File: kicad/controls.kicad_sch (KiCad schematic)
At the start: 5 parts, among them P1 Potentiometer_9mm_Vertical_Li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, P2 Potentiometer_9mm_Vertical_Li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, SW1 SW_Push_LED, SW2 SW_Push_LED, U7 ADC121C027CIMK

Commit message: reroute pcb
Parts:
- P1, P2: footprint Eurorack:Potentiometer 9mm Vertical Linear Centred -> allen-synthesis:potentiometer-9mm
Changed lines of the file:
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@@
       (effects (font (size 1.27 1.27)) (justify right) hide)
     )
-    (property "Footprint" "Eurorack:Potentiometer 9mm Vertical Linear Centred" (at 27.94 34.29 0)
+    (property "Footprint" "allen-synthesis:potentiometer-9mm" (at 27.94 34.29 0)
       (effects (font (size 1.27 1.27)) hide)
     )
@@
       (effects (font (size 1.27 1.27)) (justify right) hide)
     )
-    (property "Footprint" "Eurorack:Potentiometer 9mm Vertical Linear Centred" (at 59.69 34.29 0)
+    (property "Footprint" "allen-synthesis:potentiometer-9mm" (at 59.69 34.29 0)
       (effects (font (size 1.27 1.27)) hide)
     )

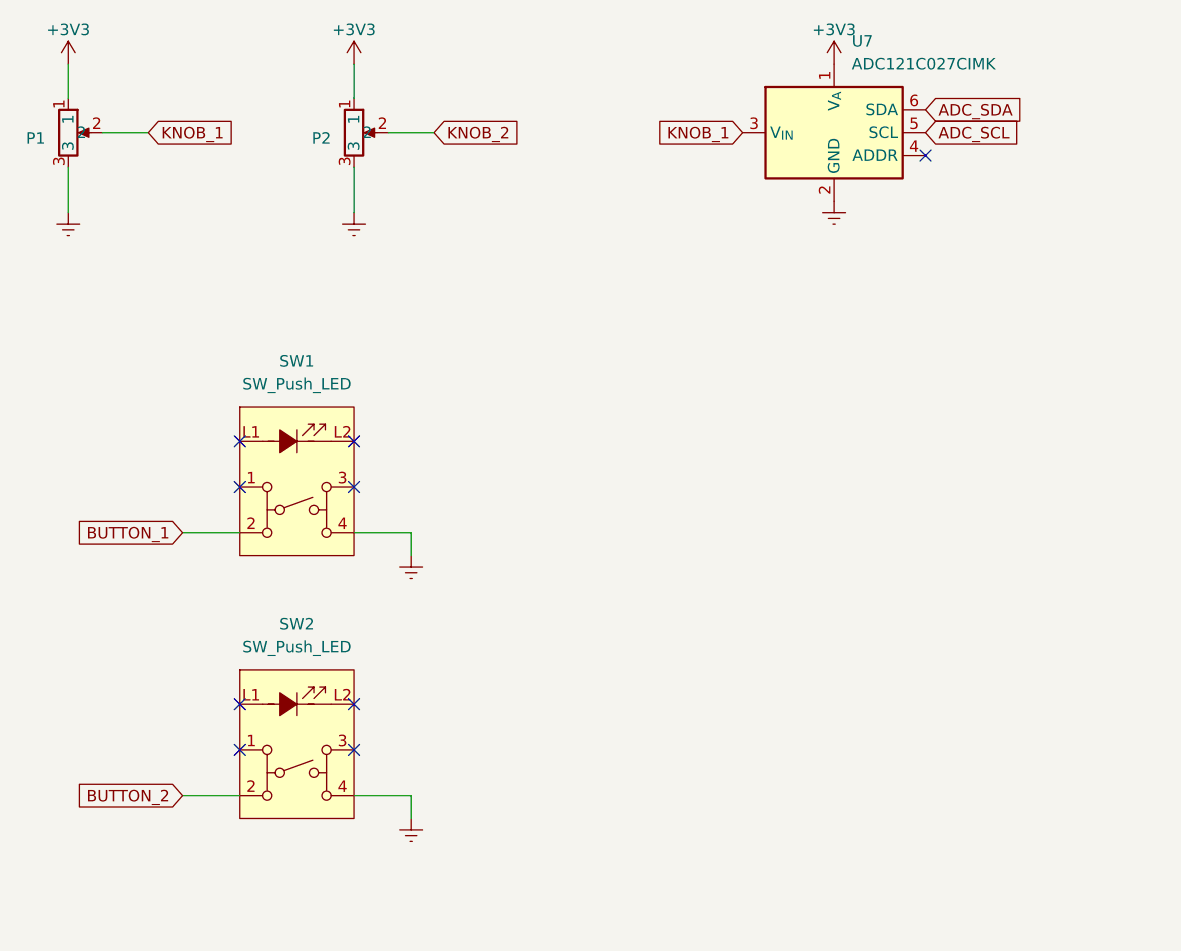
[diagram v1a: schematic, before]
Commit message: add schematic notes
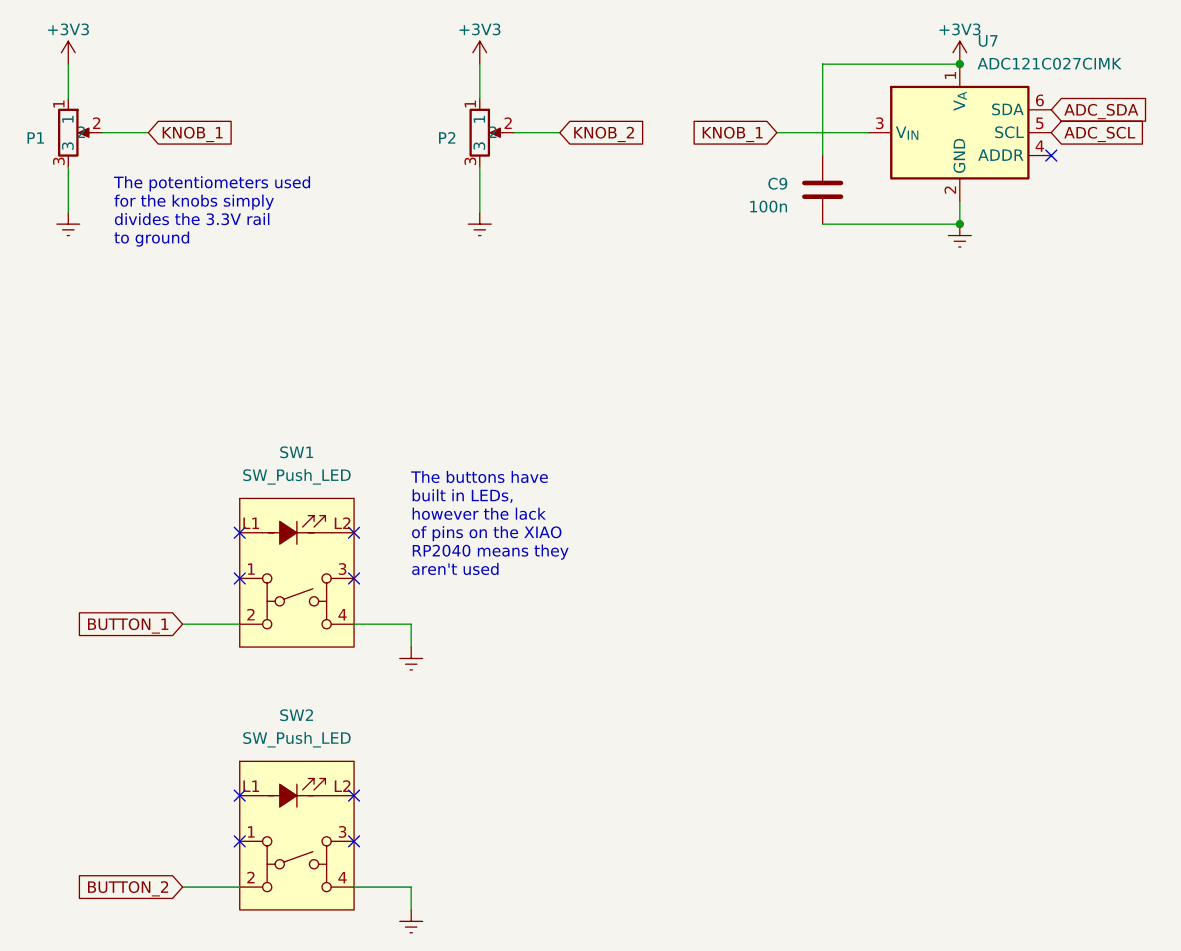
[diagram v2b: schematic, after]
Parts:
- added C9: 100n, Capacitor_SMD:C_0402_1005Metric, symbol Device:C
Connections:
- net +3V3: now also C9.1
- net Earth: now also C9.2
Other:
- note added: "The buttons have built in LEDs, however the lack of pins on the XIAO RP2040 means they aren't used"
- note added: "The potentiometers used for the knobs simply divides the 3.3V rail to ground"
- moved on the sheet: P2, SW1, SW2, U7
